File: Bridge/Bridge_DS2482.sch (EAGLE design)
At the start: 20 parts, among them Q1 BSS84, X1 3v3, X10 3v3, X11 3v3, X2 3v3, X3 GND, X4 GND, X5 GND, X6 3v3, X7 GND, X8 GND, X9 GND

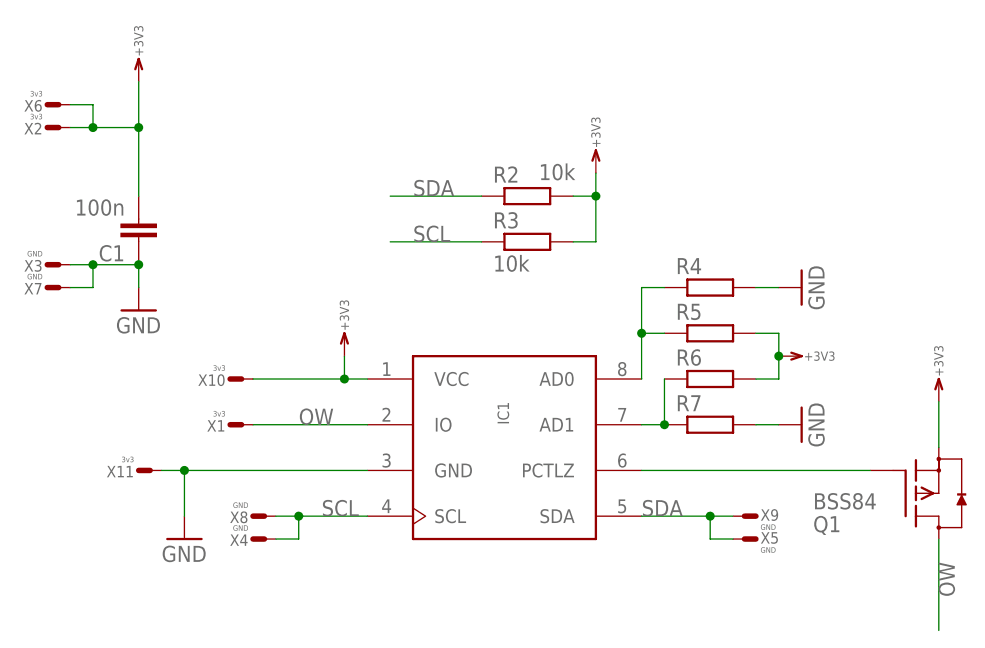
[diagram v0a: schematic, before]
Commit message: Typo correction and more elegance presentation
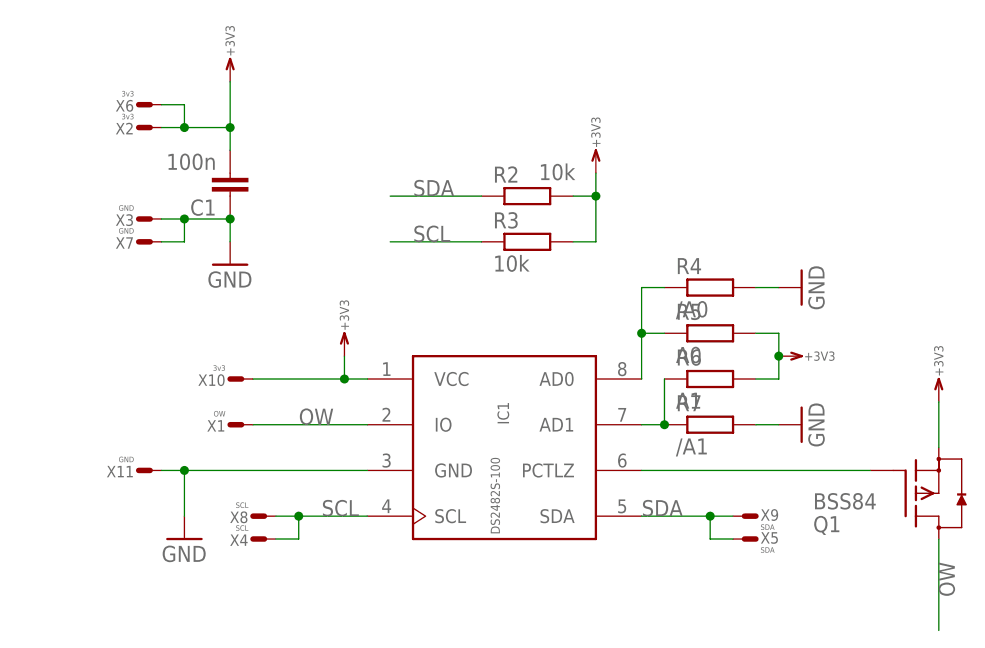
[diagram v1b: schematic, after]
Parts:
- IC1: value (none) -> DS2482S-100
- R4: value (none) -> /A0
- R5: value (none) -> A0
- R6: value (none) -> A1
- R7: value (none) -> /A1
- X1: value 3v3 -> OW
- X11: value 3v3 -> GND
- X4, X8: value GND -> SCL
- X5, X9: value GND -> SDA
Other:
- moved on the sheet: C1, X2, X3, X6, X7
